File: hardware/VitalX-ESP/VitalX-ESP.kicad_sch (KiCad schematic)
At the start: 45 parts, among them J1 ECG Probe, J2 GSR Probe, Q1 BSS138, U1 AD8232ACPZ-R7, U2 ESP32-WROOM-32U, U3 ADP160AUJZ-1.8-R7, U4 ADPD144RI-ACEZ-RL, U5 AMS1117-3.3, U6 MCP601-xOT

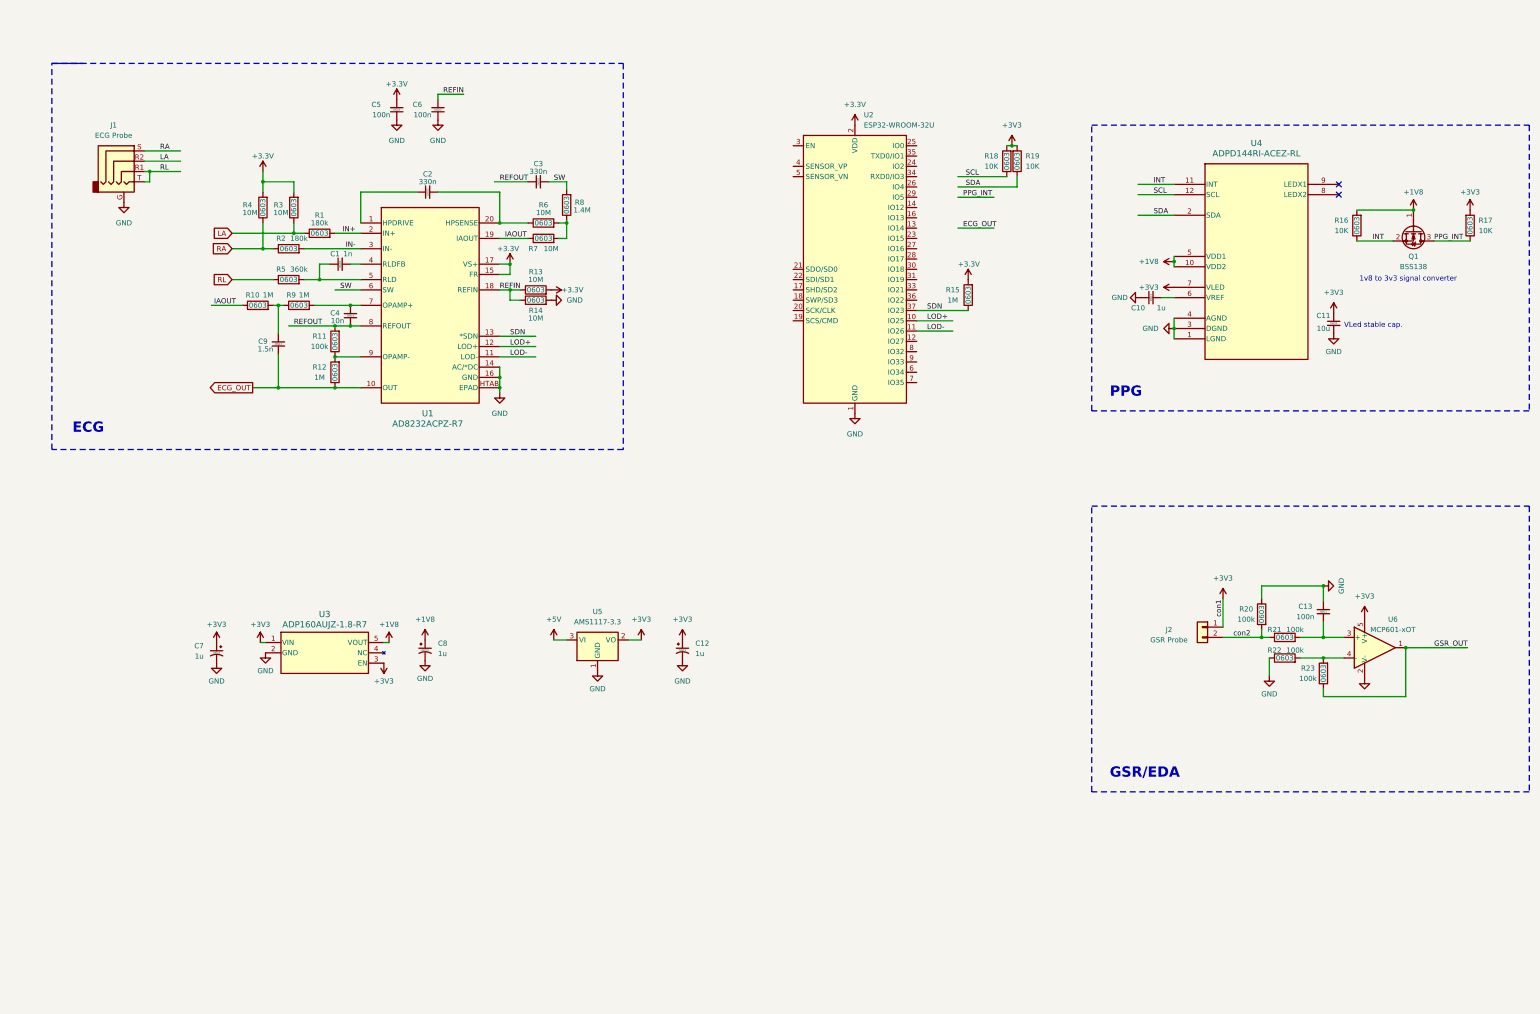
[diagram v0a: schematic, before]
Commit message: [nightly] Initial esp32-s2-wroom configuration.
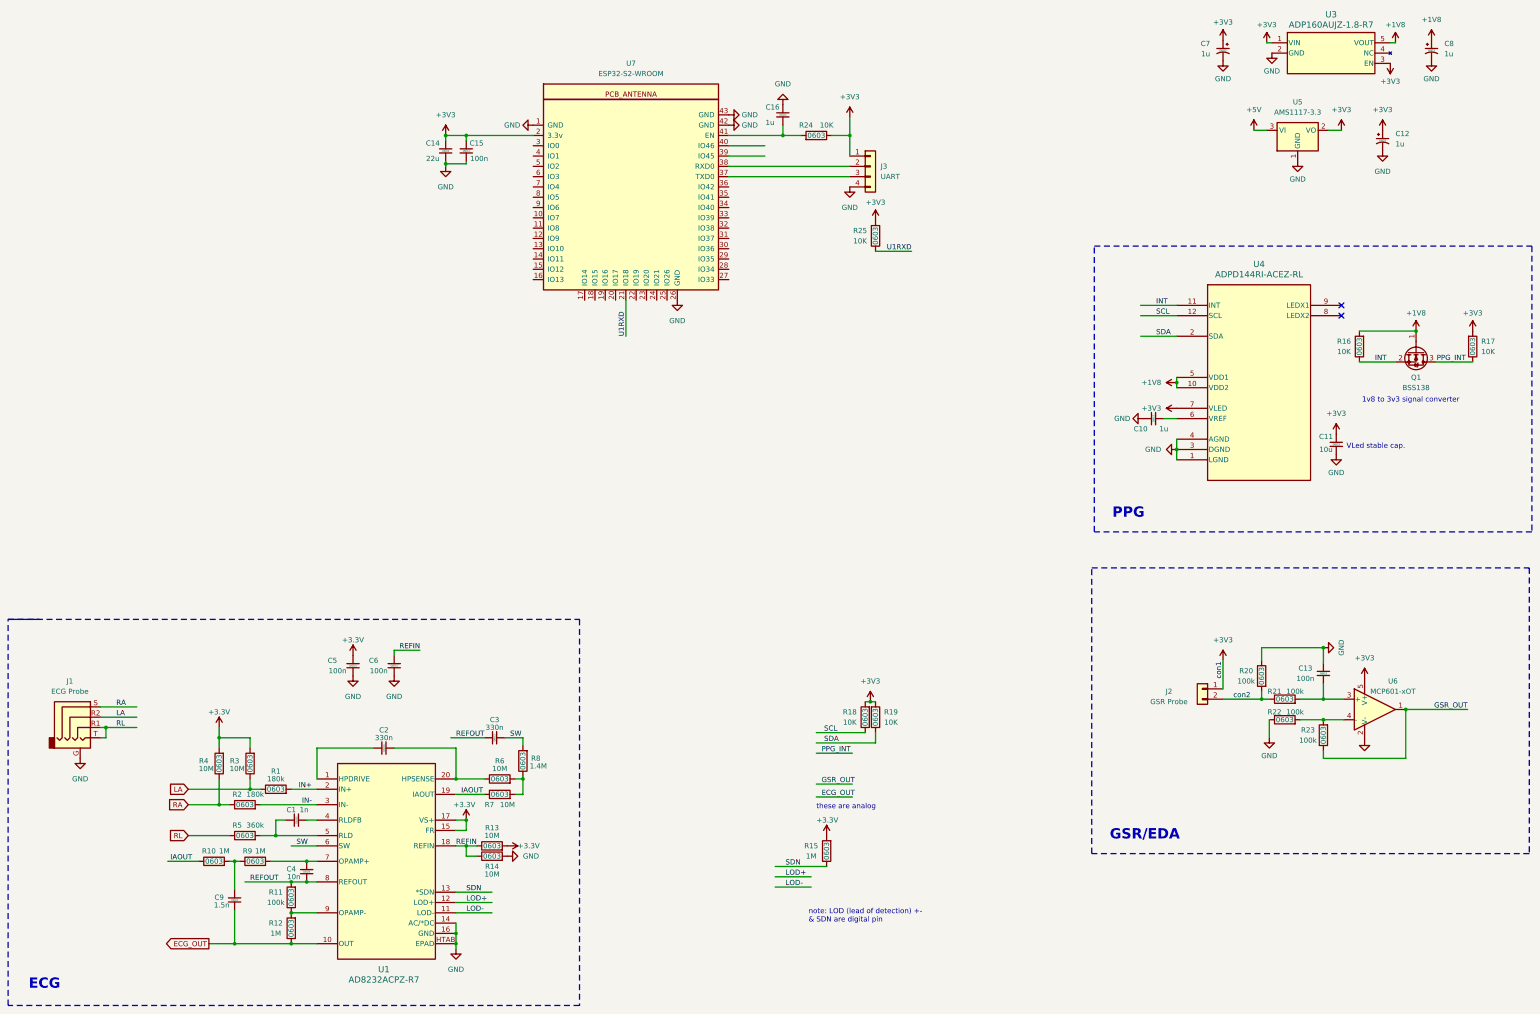
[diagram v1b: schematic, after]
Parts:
- removed U2: ESP32-WROOM-32U, RF_Module:ESP32-WROOM-32U, symbol RF_Module:ESP32-WROOM-32U
- added C14: 22u, Capacitor_SMD:C_0603_1608Metric, symbol Device:C_Small
- added C15: 100n, Capacitor_SMD:C_0603_1608Metric, symbol Device:C_Small
- added C16: 1u, Capacitor_SMD:C_0603_1608Metric, symbol Device:C_Small
- added J3: UART, symbol Connector_Generic:Conn_01x04
- added R24, R25: 10K, Resistor_SMD:R_0603_1608Metric, symbol Device:R
- added U7: ESP32-S2-WROOM, symbol ESP32-S2-WROOM:esp32-s2-wroom
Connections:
- net +3V3: now also C14.1, C15.1, J3.1 (Pin_1), R24.1, R25.2, U7.2 (3.3v)
- net GND: now also C14.2, C15.2, C16.1, J3.4 (Pin_4), U7.1 (GND), U7.26 (GND), U7.42 (GND), U7.43 (GND)
- new net: J3.3 (Pin_3), U7.37 (TXD0)
- new net: J3.2 (Pin_2), U7.38 (RXD0)
- new net: C16.2, R24.2, U7.41 (EN)
- new net U1RXD: R25.1, U7.21 (IO18)
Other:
- note added: "note: LOD (lead of detection) +- & SDN are digital pin"
- note added: "these are analog"
- moved on the sheet: C1, C10, C11, C12, C13, C2, C3, C4, C5, C6, C7, C8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
